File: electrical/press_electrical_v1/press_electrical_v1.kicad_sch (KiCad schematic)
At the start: 17 parts, among them J1 MAINS 120V 60Hz, SW1 SW_DIP_x01, SW2 RotaryEncoder_Switch, U1 34.81-9024, U2 34.81-9024

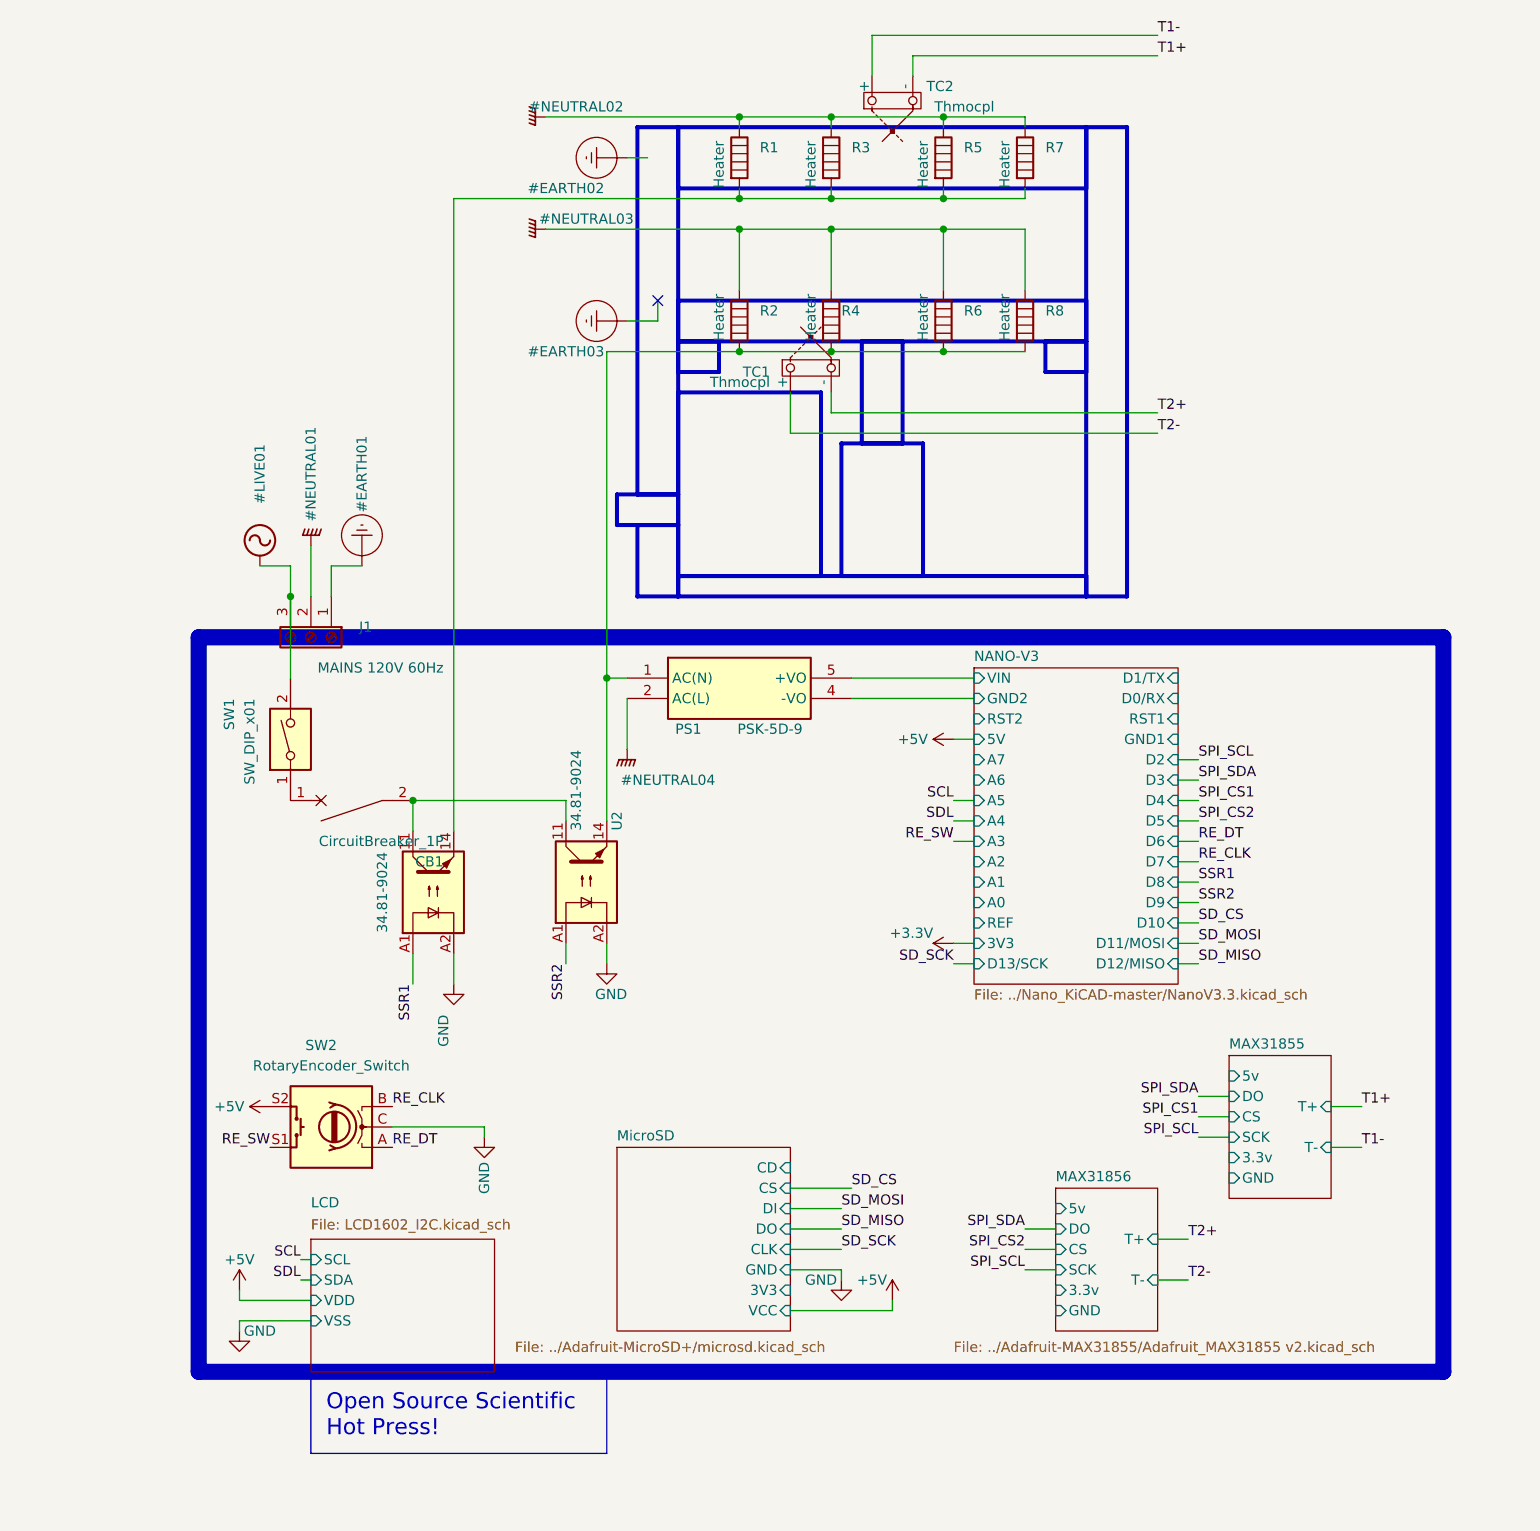
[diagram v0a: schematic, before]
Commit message: local push
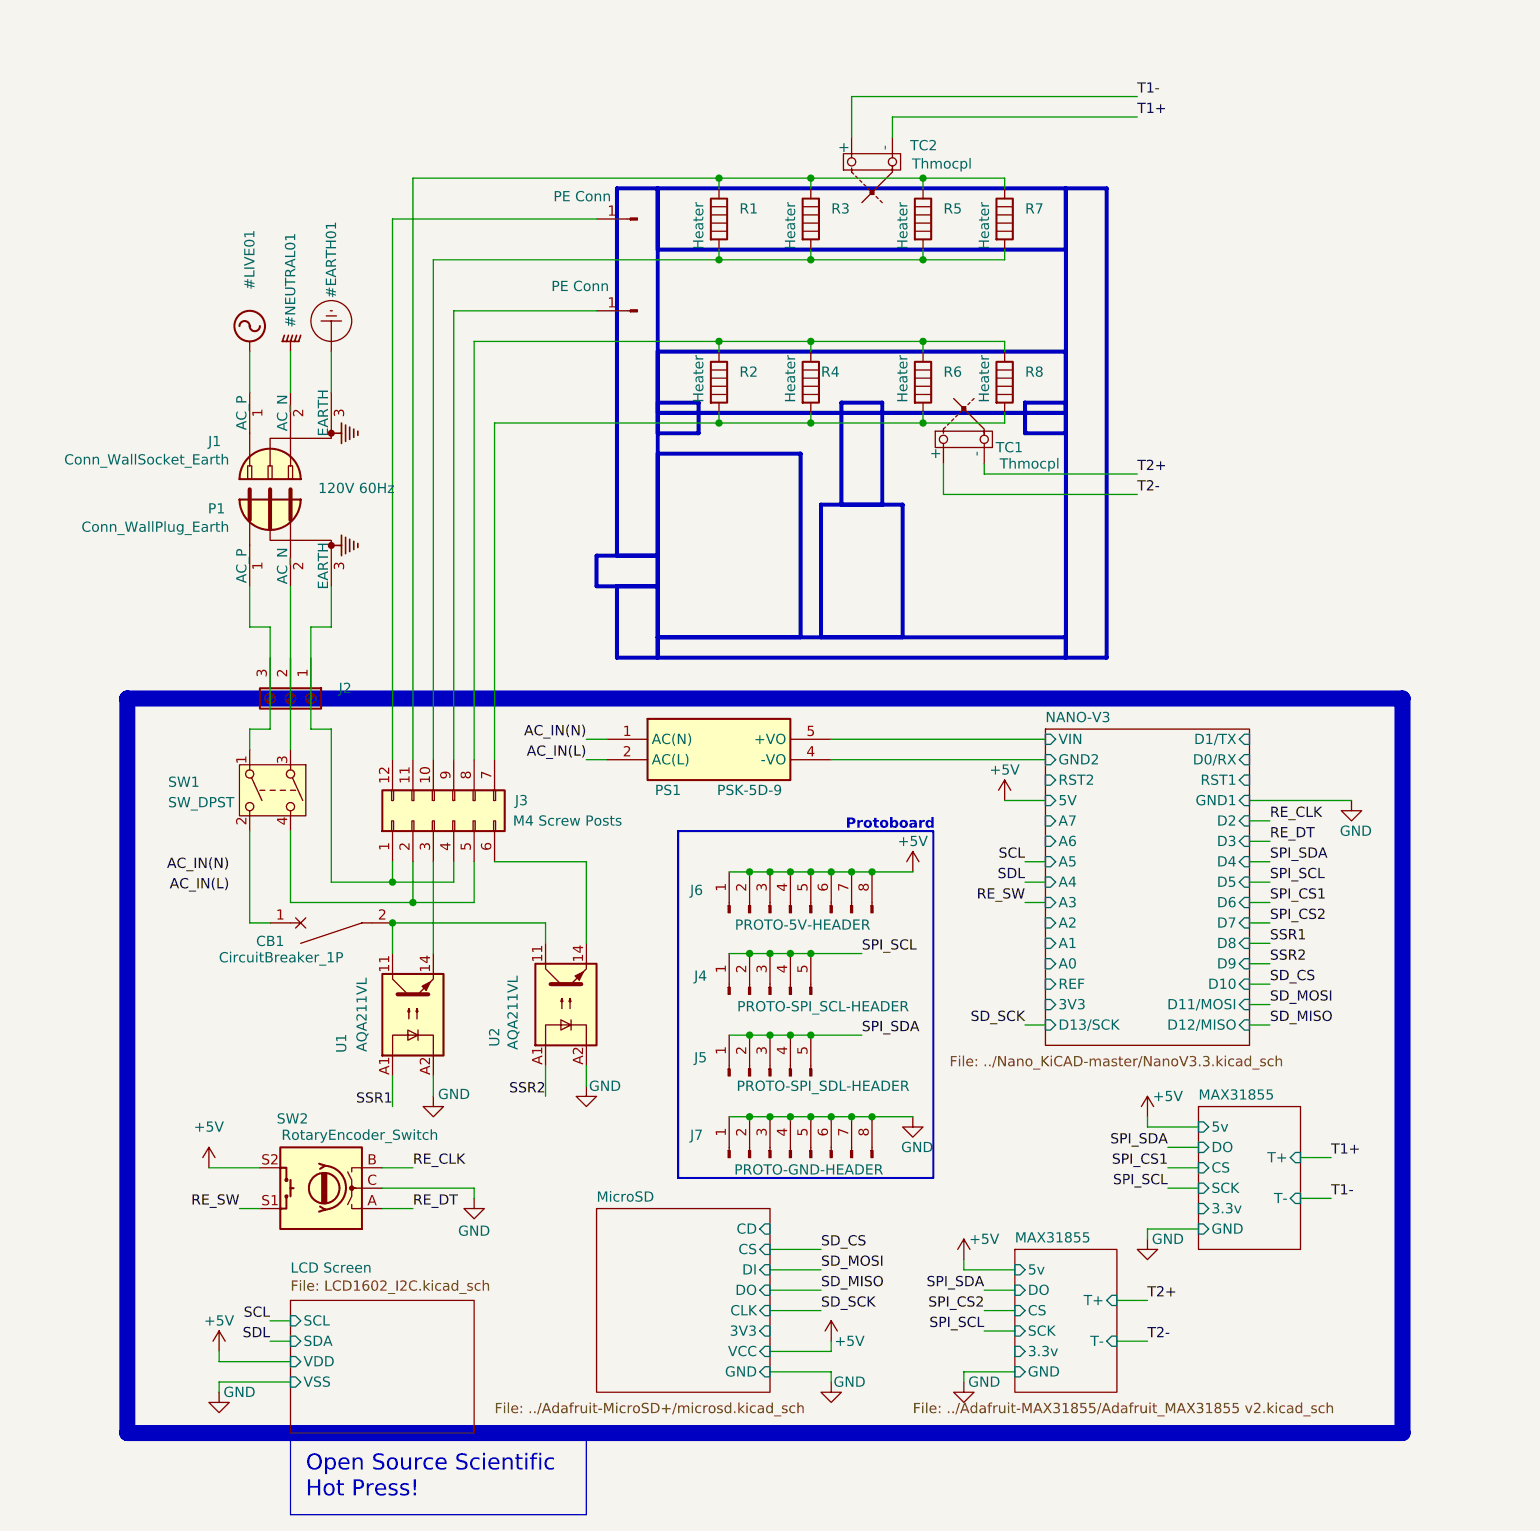
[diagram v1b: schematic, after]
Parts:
- removed SW1: SW_DIP_x01, symbol Switch:SW_DIP_x01
- added J1: Conn_WallSocket_Earth, symbol Connector:Conn_WallSocket_Earth
- added J14, J15: PE Conn, symbol Connector:Conn_01x01_Pin
- added J3: M4 Screw Posts, symbol Connector_Generic:Conn_02x06_Counter_Clockwise
- added J4: PROTO-SPI_SCL-HEADER, symbol Connector:Conn_01x05_Pin
- added J5: PROTO-SPI_SDL-HEADER, symbol Connector:Conn_01x05_Pin
- added J6: PROTO-5V-HEADER, symbol Connector:Conn_01x08_Pin
- added J7: PROTO-GND-HEADER, symbol Connector:Conn_01x08_Pin
- added P1: Conn_WallPlug_Earth, symbol Connector:Conn_WallPlug_Earth
- added SW1: SW_DPST, symbol Switch:SW_DPST
- J2: renamed from J1; value MAINS 120V 60Hz -> 120V 60Hz
- U1, U2: value 34.81-9024 -> AQA211VL
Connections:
- net +5V: now also J6.1 (Pin_1), J6.2 (Pin_2), J6.3 (Pin_3), J6.4 (Pin_4), J6.5 (Pin_5), J6.6 (Pin_6), J6.7 (Pin_7), J6.8 (Pin_8)
- net AC: now also J1.1 (AC_P); no longer J2.3 (Pin_3)
- net Earth_Protective: now also J1.3 (EARTH); no longer J2.1 (Pin_1)
- net GND: now also J7.1 (Pin_1), J7.2 (Pin_2), J7.3 (Pin_3), J7.4 (Pin_4), J7.5 (Pin_5), J7.6 (Pin_6), J7.7 (Pin_7), J7.8 (Pin_8)
- net GNDPWR: now also J1.2 (AC_N); no longer J2.2 (Pin_2), PS1.2 (AC(L)), R1.1, R2.1, R3.1, R4.1, R5.1, R6.1, R7.1, R8.1
- net SPI_SCL: now also J4.1 (Pin_1), J4.2 (Pin_2), J4.3 (Pin_3), J4.4 (Pin_4), J4.5 (Pin_5)
- net SPI_SDA: now also J5.1 (Pin_1), J5.2 (Pin_2), J5.3 (Pin_3), J5.4 (Pin_4), J5.5 (Pin_5)
- net at R2.2, R4.2, R6.2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: now also J3.7 (Pin_7); no longer PS1.1 (AC(N)), U2.14
- net at R1.2, R3.2, R5.2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: now also J3.10 (Pin_10); no longer U1.14
- net at CB1.1: now also SW1.2
- new net: P1.1 (AC_P), SW1.1
- new net: P1.2 (AC_N), SW1.3
- new net: J3.2 (Pin_2), J3.5 (Pin_5), SW1.4
- new net: J3.1 (Pin_1), J3.4 (Pin_4), P1.3 (EARTH)
- new net: J3.11 (Pin_11), R1.1, R3.1, R5.1, R7.1
- new net: J15.1 (Pin_1), J3.12 (Pin_12)
- new net: J3.3 (Pin_3), U1.14
- new net: J3.6 (Pin_6), U2.14
- new net: J3.8 (Pin_8), R2.1, R4.1, R6.1, R8.1
- new net: J14.1 (Pin_1), J3.9 (Pin_9)
- new net AC_IN(L): PS1.2 (AC(L))
- new net AC_IN(N): PS1.1 (AC(N))
- no-connect marks 1 -> 0
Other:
- sheet LCD renamed LCD Screen
- removed sheet MAX31856
- note added: "Protoboard"
- moved on the sheet: CB1, J2, PS1, R1, R2, R3, R4, R5, R6, R7, R8, SW2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
